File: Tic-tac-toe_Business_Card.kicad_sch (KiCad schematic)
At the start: 76 parts, among them J1 USB_C_Receptacle_USB2.0_14P, J2 Conn_01x04, SW1 SW_Push, SW2 SW_Push, SW3 SW_Push, U1 MCP1700x-330xxTT, U3 RP2040, U4 W25Q16JVUXIQ TR, Y1 12 MHz

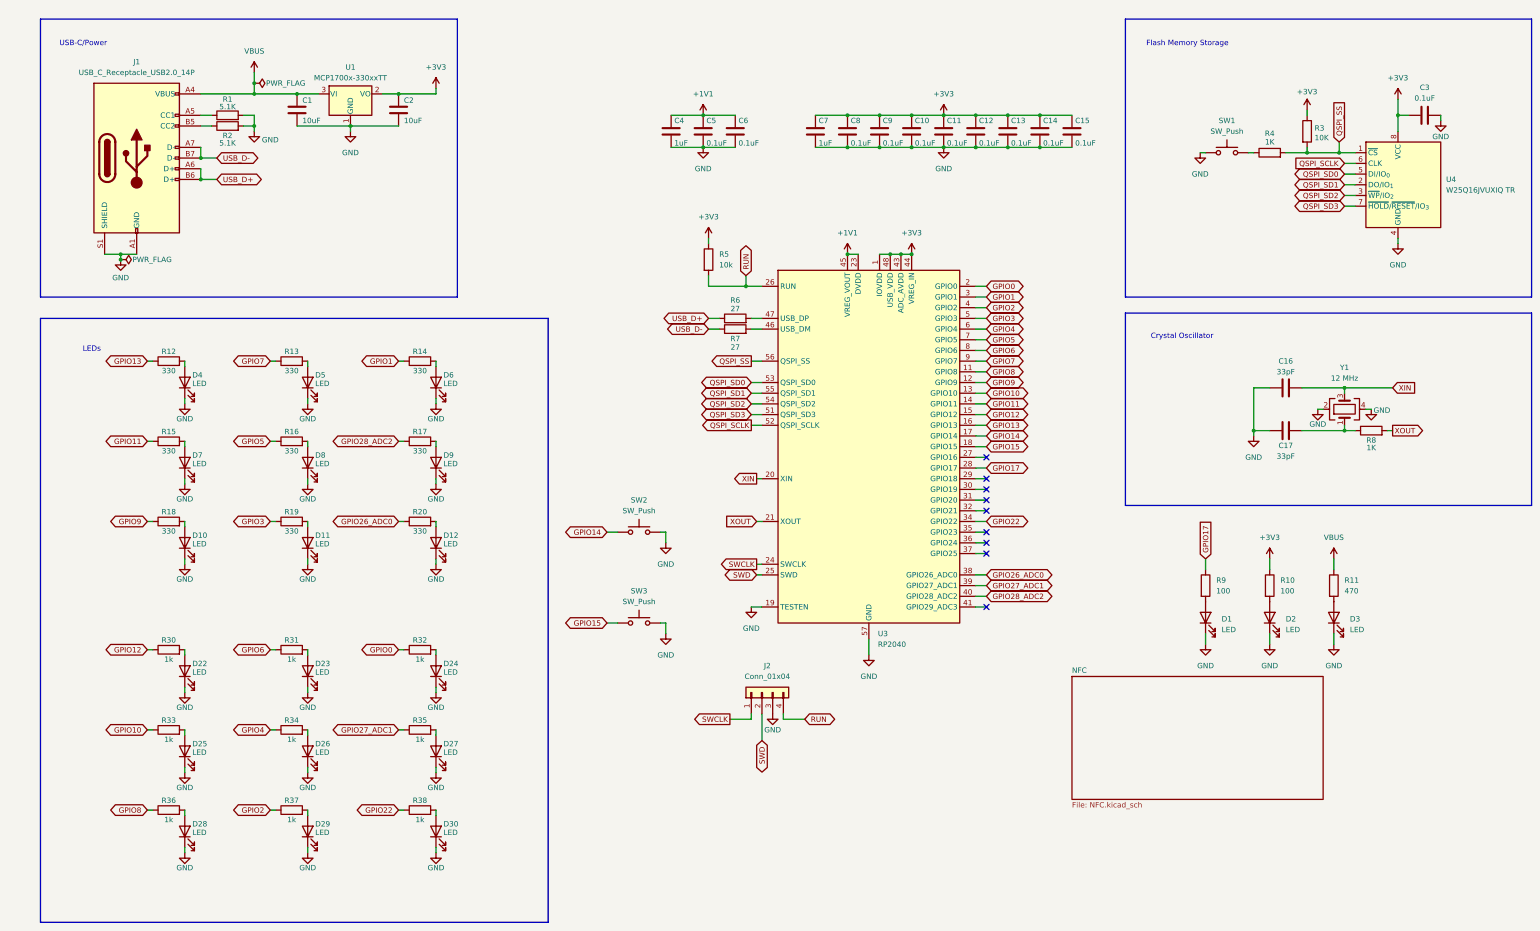
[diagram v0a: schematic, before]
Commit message: Update Readme
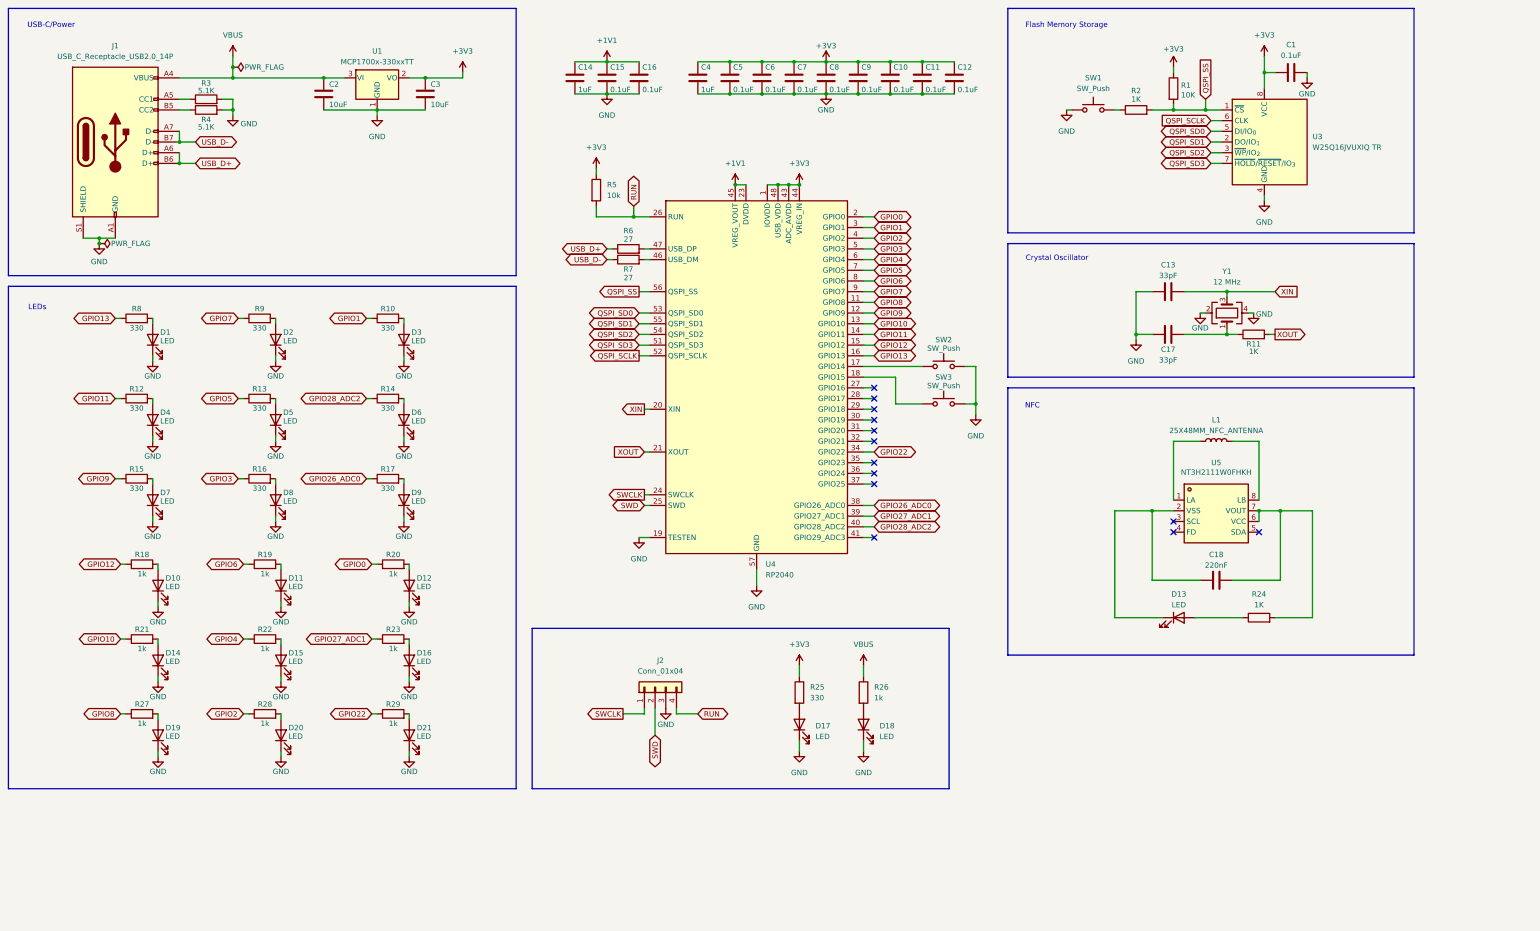
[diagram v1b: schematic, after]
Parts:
- removed D1: LED, LED_SMD:LED_0603_1608Metric, symbol Device:LED
- removed R9: 100, Resistor_SMD:R_0402_1005Metric, symbol Device:R
- added C18: 220nF, Capacitor_SMD:C_0603_1608Metric, symbol Device:C
- added D13: LED, LED_SMD:LED_0402_1005Metric, symbol Device:LED
- added L1: 25X48MM_NFC_ANTENNA, NFC_Tic_Tac_Toe:25X48MM_NFC_ANTENNA, symbol Device:L
- added R24: 1K, Resistor_SMD:R_0402_1005Metric, symbol Device:R
- added U5: NT3H2111W0FHKH, NFC_Tic_Tac_Toe:XQFN-8_L1.6-W1.6-P0.50-BL_NT3H2111W0FHKH, symbol CyberCard:NT3H2111W0FHKH
- R25: renamed from R10; value 100 -> 330
- R26: renamed from R11; value 470 -> 1k
- renumbered C3 to C1, C13 to C10, C14 to C11, C15 to C12, C16 to C13, C4 to C14, C5 to C15, C6 to C16, C1 to C2, C2 to C3, C7 to C4, C8 to C5, C9 to C6, C10 to C7, C11 to C8, C12 to C9, D4 to D1, D22 to D10, D23 to D11, D24 to D12, D25 to D14, D26 to D15, D27 to D16, D2 to D17, D3 to D18, D28 to D19, D5 to D2, D29 to D20, D30 to D21, D6 to D3, D7 to D4, D8 to D5, D9 to D6, D10 to D7, D11 to D8, D12 to D9, R3 to R1, R14 to R10, R8 to R11, R15 to R12, R16 to R13, R17 to R14, R18 to R15, R19 to R16, R20 to R17, R30 to R18, R31 to R19, R4 to R2, R32 to R20, R33 to R21, R34 to R22, R35 to R23, R36 to R27, R37 to R28, R38 to R29, R1 to R3, R2 to R4, R12 to R8, R13 to R9, U4 to U3, U3 to U4
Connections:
- net GPIO14: no longer names the net of SW2.1, U4.17 (GPIO14)
- net GPIO15: no longer names the net of SW3.1, U4.18 (GPIO15)
- net GPIO17: no longer names the net of U4.28 (GPIO17)
- new net: C18.1, D13.1 (K), U5.2 (VSS)
- new net: C18.2, R24.2, U5.6 (VCC), U5.7 (VOUT)
- new net: D13.2 (A), R24.1
- new net: L1.1, U5.1 (LA)
- new net: L1.2, U5.8 (LB)
- no-connect marks 9 -> 13
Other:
- removed sheet NFC
- note added: "NFC"
- title: (none) -> Tic-tac-toe Business Card V2
- moved on the sheet: C1, C10, C11, C12, C13, C14, C15, C16, C17, C2, C3, C4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
